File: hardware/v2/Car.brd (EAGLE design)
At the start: 84 x 56 mm, 63 parts

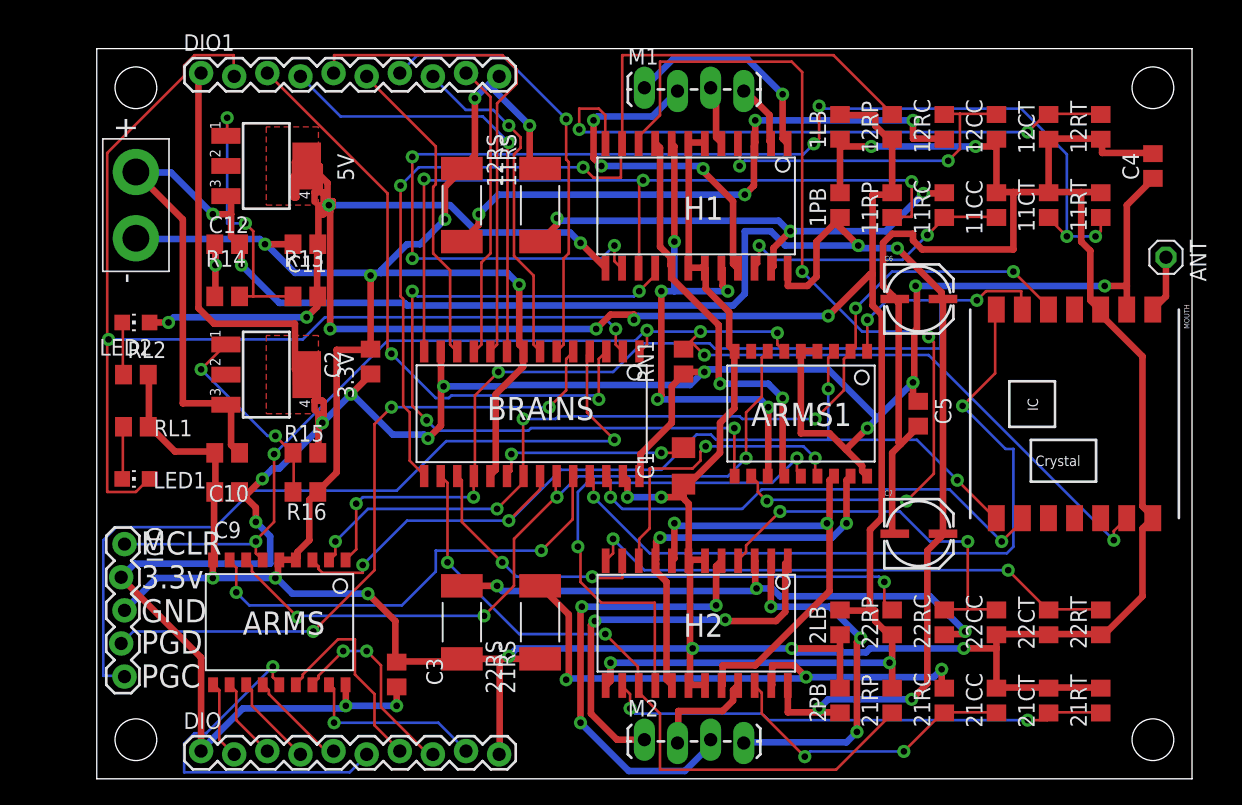
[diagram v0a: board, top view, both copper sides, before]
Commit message: Completed Rev.A of v2 hardware.
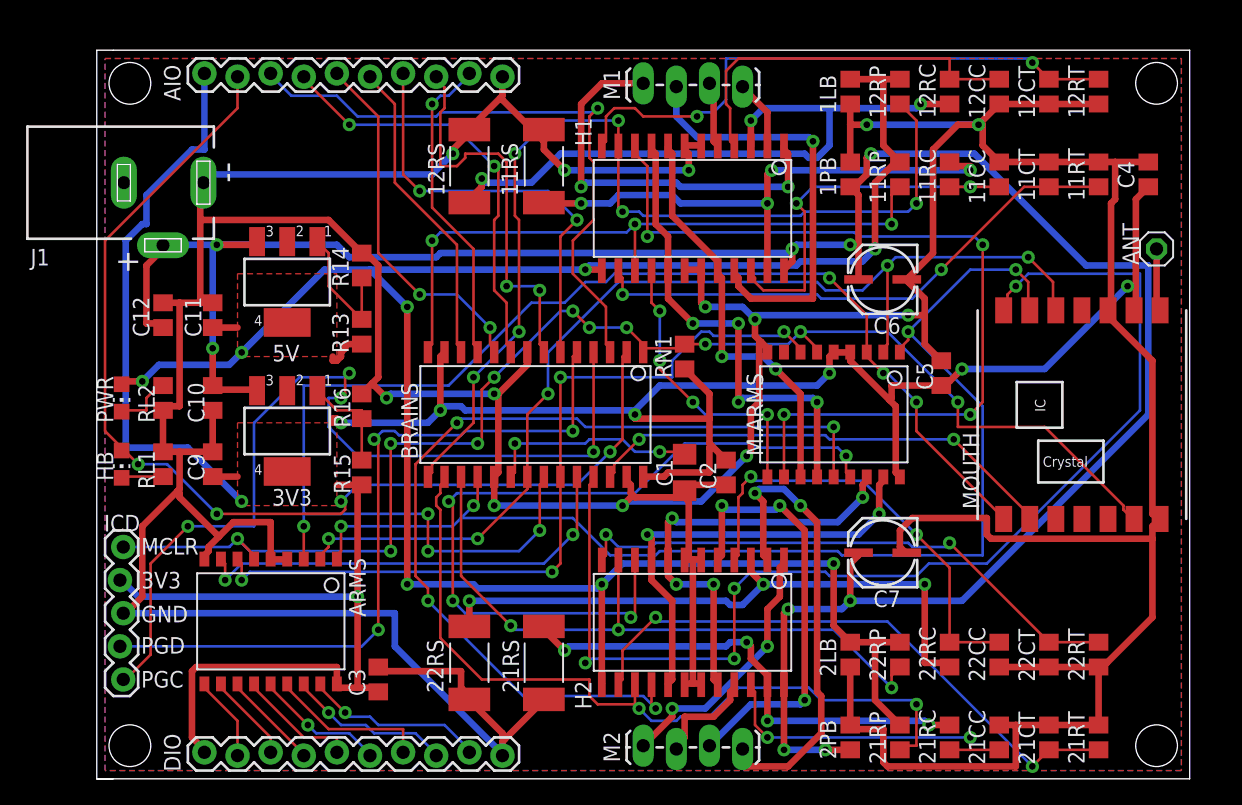
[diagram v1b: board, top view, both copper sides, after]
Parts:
- removed 3.3V: 317EMP, linear:SOT223
- removed ARMS1: MCP23S08, microchip:SO-18W
- removed DIO1: (no value), SparkFun-Connectors:1X10_LOCK
- removed LED1, LED2: (no value), led:CHIP-LED0805
- removed POW: (no value), SparkFun-Connectors:1X02_XTRA_BIG
- added 3V3: 317EMP, linear:SOT223
- added AIO: (no value), SparkFun-Connectors:1X10_LOCK
- added HB, PWR: (no value), led:CHIP-LED0805
- added J1: (no value), con-jack:DCJ0303
- added M.ARMS: MCP23S08, microchip:SO-18W
- moved C2 28.6 mm to (48.3, 23.5), turned to 270 degrees
- moved R14 10.6 mm to (20.3, 39.4), turned to 270 degrees
- moved 5V 9.04 mm to (14.6, 38.1), turned to 180 degrees
- moved C11 8.95 mm to (8.89, 35.6), turned to 90 degrees
- moved R16 7.87 mm to (20.3, 28.6), turned to 270 degrees
- moved C12 7.33 mm to (5.08, 35.6), turned to 90 degrees
- moved R13 5.10 mm to (20.3, 34.3), turned to 270 degrees
- moved R15 4.57 mm to (20.3, 23.5), turned to 270 degrees
- moved C10 4.35 mm to (8.89, 29.2), turned to 270 degrees
- moved C5 3.58 mm to (64.8, 31.1), turned to 90 degrees
- moved RL1 3.54 mm to (5.08, 24.1), turned to 90 degrees
- moved C7 3.26 mm to (60.3, 17.1), turned to 180 degrees
- moved 22RS 3.16 mm to (28.6, 8.89)
- moved 21RS 3.12 mm to (34.3, 8.89)
- moved 12RS 3.04 mm to (28.6, 47.0)
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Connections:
- net +12V: now also 3V3.3, J1.2; no longer 3.3V.3, POW.1
- net +3V3: now also 3V3.4, AIO.1, M.ARMS.18, M.ARMS.4, M.ARMS.5; no longer 3.3V.4, ARMS1.18, ARMS1.4, ARMS1.5, DIO1.1
- net +5V: now also PWR.A; no longer LED2.A
- net GND: now also AIO.10, J1.1, M.ARMS.9; no longer ARMS1.9, DIO1.10, POW.2
- net N$20: now also 3V3.1; no longer 3.3V.1
- net N$23: now also M.ARMS.12; no longer ARMS1.12
- net N$25: now also M.ARMS.2; no longer ARMS1.2
- net N$26: now also M.ARMS.3; no longer ARMS1.3
- net N$29: now also AIO.4; no longer DIO1.4
- net N$32: now also AIO.5; no longer DIO1.5
- net N$36: now also M.ARMS.7; no longer ARMS1.7
- net N$45: now also AIO.2, HB.A; no longer DIO1.2, LED1.A
- net N$46: now also HB.C; no longer LED1.C
- net N$53: now also AIO.3; no longer DIO1.3
- net N$54: now also AIO.7; no longer DIO1.7
- net N$55: now also AIO.8; no longer DIO1.8
- net N$56: now also M.ARMS.13; no longer ARMS1.13
- net N$57: now also AIO.6; no longer DIO1.6
- net N$59: now also AIO.9; no longer DIO1.9
- net N$60: now also M.ARMS.16; no longer ARMS1.16
- net N$61: now also M.ARMS.17; no longer ARMS1.17
- net N$62: now also M.ARMS.10; no longer ARMS1.10
- net N$63: now also M.ARMS.11; no longer ARMS1.11
- net N$65: now also PWR.C; no longer LED2.C
- net N$66: now also M.ARMS.14; no longer ARMS1.14
- net N$67: now also M.ARMS.15; no longer ARMS1.15
- net N$7: now also M.ARMS.1; no longer ARMS1.1
- net VCCIO: now also M.ARMS.6; no longer ARMS1.6
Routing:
- net N$41: track 92.7 -> 42.2 mm, vias 7 -> 2
- net GND: track 419.5 -> 470.0 mm, vias 18 -> 13
- net N$67: track 23.1 -> 60.9 mm, vias 2 -> 4
- net N$62: track 58.1 -> 22.3 mm
- net N$26: track 71.8 -> 107.4 mm, vias 4 -> 7
- net N$22: track 57.2 -> 91.2 mm, vias 2 -> 4
- net N$66: track 39.1 -> 71.3 mm, vias 2 -> 4
- net +5V: track 201.1 -> 171.4 mm, vias 10 -> 8
- net +12V: track 161.3 -> 183.0 mm, vias 6 -> 9
- net N$50: track 27.7 -> 10.1 mm
- net N$2: track 16.6 -> 31.2 mm, vias 1 -> 2
- net N$7: track 79.6 -> 92.4 mm, vias 5 -> 4
- net +3V3: track 230.0 -> 218.4 mm, vias 13 -> 8
- net N$8: track 31.2 -> 20.2 mm
- net N$30: track 61.8 -> 51.2 mm
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- added copper zone on layer 1, net GND
- added copper zone on layer 16, net GND
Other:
- board size 84 x 56 mm -> 83.8 x 55.9 mm
- board text added: "--"
- board text added: "3V3"
- board text removed: "-"
- board text removed: "3.3v"
